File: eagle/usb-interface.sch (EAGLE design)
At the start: 16 parts

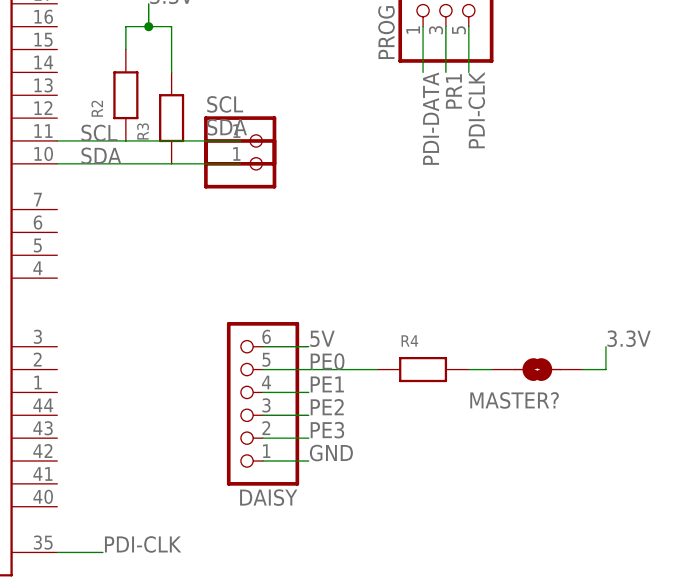
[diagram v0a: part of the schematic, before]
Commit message: major rework of usb interface board - dropped Y by 5mm, cleaned routing, added better mounting.
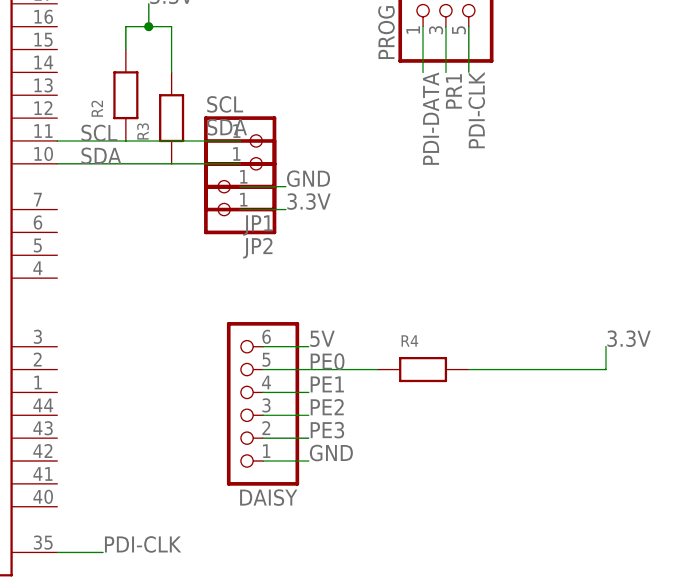
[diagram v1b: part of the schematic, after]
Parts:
- removed MASTER?: SOLDERJUMPERN, SparkFun:SOLDERJUMPERNC
- added JP1, JP2: (no value), nonolith:HEADER-1X12MM
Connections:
- removed net PE0-PULL: MASTER?.2, R4.2
- net 3.3V: now also JP2.1, R4.2; no longer MASTER?.1
- net GND: now also JP1.1
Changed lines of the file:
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@@
 <part name="DAISY" library="nonolith" deviceset="HEADER-1X6" device="2MM"/>
 <part name="R4" library="nonolith" deviceset="RESISTOR" device="0603"/>
-<part name="MASTER?" library="SparkFun" deviceset="SOLDERJUMPER" device="NC" value="SOLDERJUMPERN"/>
 <part name="SCL" library="nonolith" deviceset="HEADER-1X1" device="2MM"/>
 <part name="SDA" library="nonolith" deviceset="HEADER-1X1" device="2MM"/>
+<part name="JP1" library="nonolith" deviceset="HEADER-1X1" device="2MM"/>
+<part name="JP2" library="nonolith" deviceset="HEADER-1X1" device="2MM"/>
 </parts>
 <sheets>
@@
 <instance part="DAISY" gate="A" x="127" y="20.32" rot="R180"/>
 <instance part="R4" gate="G$1" x="147.32" y="22.86"/>
-<instance part="MASTER?" gate="1" x="160.02" y="22.86" smashed="yes" rot="R180">
-<attribute name="NAME" x="162.56" y="20.32" size="1.778" layer="95" rot="R180"/>
-</instance>
 <instance part="SCL" gate="G$1" x="129.54" y="48.26"/>
 <instance part="SDA" gate="G$1" x="129.54" y="45.72"/>
+<instance part="JP1" gate="G$1" x="124.46" y="43.18" rot="R180"/>
+<instance part="JP2" gate="G$1" x="124.46" y="40.64" rot="R180"/>
 </instances>
 <busses>
@@
 <wire x1="129.54" y1="12.7" x2="134.62" y2="12.7" width="0" layer="91"/>
 <label x="134.62" y="12.7" size="1.778" layer="95"/>
+</segment>
+<segment>
+<pinref part="JP1" gate="G$1" pin="1"/>
+<wire x1="127" y1="43.18" x2="132.08" y2="43.18" width="0" layer="91"/>
+<label x="132.08" y="43.18" size="1.778" layer="95"/>
 </segment>
 </net>
@@
 </segment>
 <segment>
-<pinref part="MASTER?" gate="1" pin="1"/>
-<wire x1="165.1" y1="22.86" x2="167.64" y2="22.86" width="0" layer="91"/>
 <wire x1="167.64" y1="22.86" x2="167.64" y2="25.4" width="0" layer="91"/>
 <label x="167.64" y="25.4" size="1.778" layer="95"/>
+<pinref part="R4" gate="G$1" pin="2"/>
+<wire x1="167.64" y1="22.86" x2="152.4" y2="22.86" width="0" layer="91"/>
+</segment>
+<segment>
+<pinref part="JP2" gate="G$1" pin="1"/>
+<wire x1="127" y1="40.64" x2="132.08" y2="40.64" width="0" layer="91"/>
+<label x="132.08" y="40.64" size="1.778" layer="95"/>
 </segment>
 </net>
@@
 </segment>
 </net>
-<net name="PE0-PULL" class="0">
-<segment>
-<pinref part="R4" gate="G$1" pin="2"/>
-<pinref part="MASTER?" gate="1" pin="2"/>
-<wire x1="152.4" y1="22.86" x2="154.94" y2="22.86" width="0" layer="91"/>
-</segment>
-</net>
